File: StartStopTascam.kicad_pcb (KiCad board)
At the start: 2 copper layers, 19 parts, among them J1 Jack_LJB0670, J2 Jack_LJB0670, J3 DB9_Male, P1 CONN_02X03, U1 MAX232

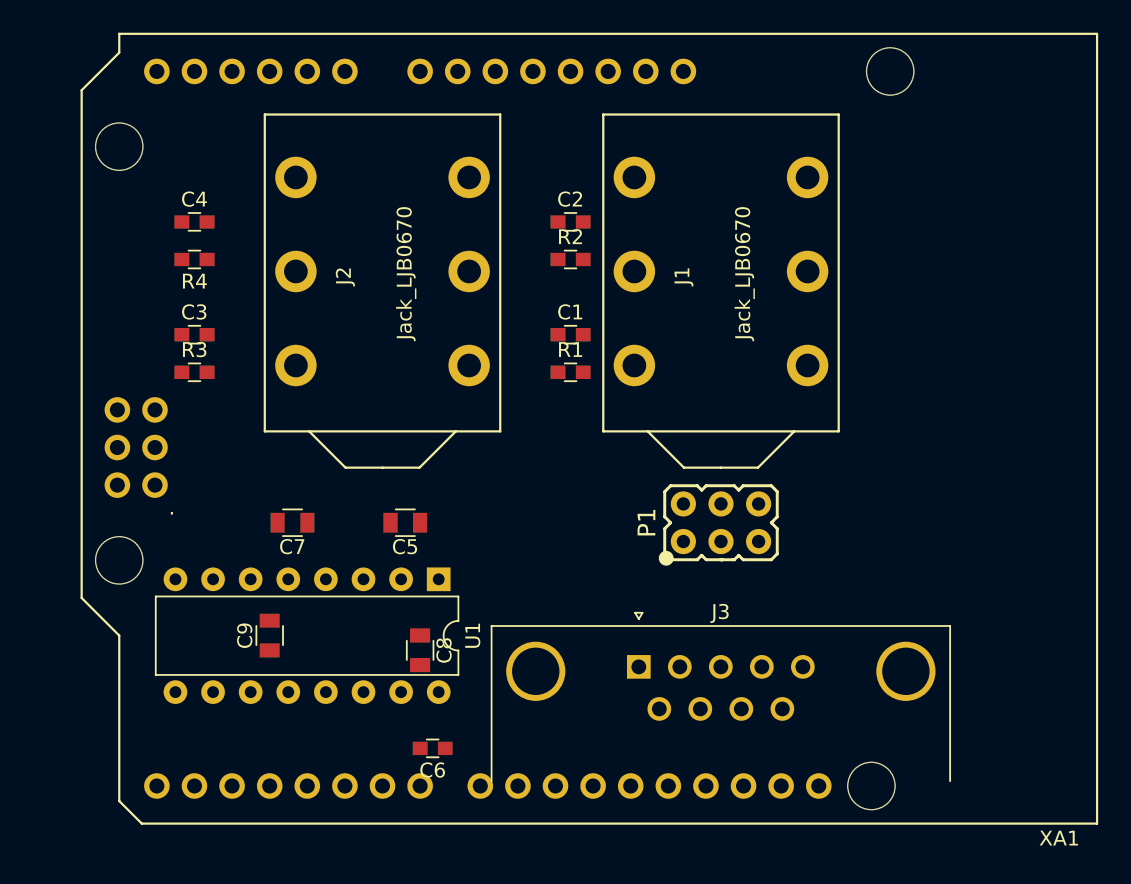
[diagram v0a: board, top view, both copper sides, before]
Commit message: kicad
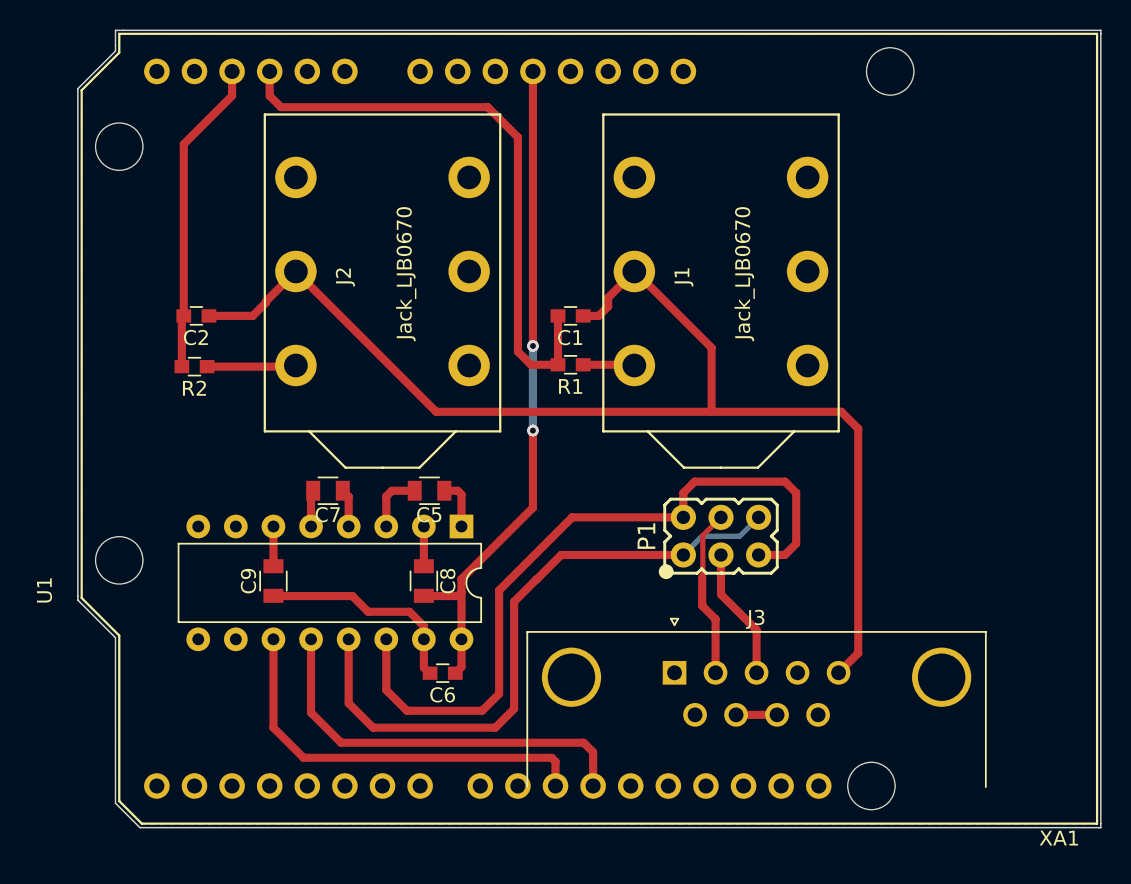
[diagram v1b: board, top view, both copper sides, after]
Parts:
- removed the C2 at (99.1, 45.7)
- removed C4: 100N-X7R_50V#0603, D&R_Passive:C_0603
- removed R3, R4: R, D&R_Passive:C_0603
- C1: value 100N-X7R_50V#0603 -> 100N-X7R_50V#0603-D&R_Passive
- C2: renamed from C3; value 100N-X7R_50V#0603 -> 100N-X7R_50V#0603-D&R_Passive
- R1, R2: value R -> 4k7
- moved R2 26.4 mm to (73.7, 55.5), turned to 180 degrees
- moved C6 5.12 mm to (90.4, 76.2)
- moved C8 4.69 mm to (89.2, 70.0)
- moved U1 3.88 mm to (91.7, 66.3)
- moved C9 3.69 mm to (79.0, 70.0)
- moved C7 3.23 mm to (82.7, 63.9)
- moved C5 2.71 mm to (89.5, 63.9)
- moved J3 2.45 mm to (106.1, 76.2)
- moved C2 1.28 mm to (73.8, 52.1), turned to 180 degrees
- moved C1 1.27 mm to (99.1, 52.1), turned to 180 degrees
- moved P1 0.91 mm to (109.2, 66.9)
- moved R1 0.51 mm to (99.1, 55.4), turned to 180 degrees
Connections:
- C1 pad 2: Net-(C1-Pad2) -> Net-(XA1-PadA2)
- C2 pad 2: Net-(C3-Pad2) -> Net-(XA1-PadA3)
- J1 pad 3: Net-(J1-Pad3) -> GND
- J1 pad 5: GND -> unconnected-(J1-Pad5)
- J2 pad 3: Net-(J2-Pad3) -> GND
- J2 pad 5: GND -> unconnected-(J2-Pad5)
- J3 pad 7: unconnected-(J3-Pad7) -> Net-(J3-Pad7)
- J3 pad 8: unconnected-(J3-Pad8) -> Net-(J3-Pad7)
- R1 pad 2: Net-(C1-Pad2) -> Net-(XA1-PadA2)
- R2 pad 1: Net-(J1-Pad3) -> Net-(J2-Pad1)
- R2 pad 2: Net-(C2-Pad1) -> Net-(XA1-PadA3)
- U1 pad 11: Net-(U1-Pad11) -> Net-(XA1-PadD10)
- U1 pad 12: unconnected-(U1-Pad12) -> Net-(XA1-PadD11)
- XA1 pad A0: Net-(C4-Pad1) -> unconnected-(XA1-PadA0)
- XA1 pad A1: Net-(C3-Pad2) -> unconnected-(XA1-PadA1)
- XA1 pad A2: Net-(C2-Pad1) -> Net-(XA1-PadA2)
- XA1 pad A3: Net-(C1-Pad2) -> Net-(XA1-PadA3)
- XA1 pad D10: unconnected-(XA1-PadD10) -> Net-(XA1-PadD10)
- XA1 pad D11: unconnected-(XA1-PadD11) -> Net-(XA1-PadD11)
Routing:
- net GND: track 0.00 -> 97.8 mm
- net Net-(P1-Pad2): track 0.00 -> 49.8 mm
- net VCC: track 0.00 -> 47.1 mm, vias 0 -> 2
- net Net-(P1-Pad1): track 0.00 -> 42.8 mm
- net Net-(XA1-PadA2): track 0.00 -> 40.4 mm
- net Net-(XA1-PadD10): track 0.00 -> 27.6 mm
- net Net-(XA1-PadD11): track 0.00 -> 27.4 mm
- net Net-(XA1-PadA3): track 0.00 -> 21.5 mm
- net Net-(J3-Pad2): track 0.00 -> 11.4 mm
- net Net-(J3-Pad3): track 0.00 -> 8.95 mm
- net Net-(J2-Pad1): track 0.00 -> 6.03 mm
- net Net-(C5-Pad2): track 0.00 -> 4.11 mm
- net Net-(J1-Pad1): track 0.00 -> 3.55 mm
- net Net-(C5-Pad1): track 0.00 -> 3.42 mm
- net Net-(J3-Pad7): track 0.00 -> 2.77 mm
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- added copper zone on B.Cu, net GND
- added copper zone on F.Cu, net GND
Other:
- board outline added: 69.1 x 53.8 mm
